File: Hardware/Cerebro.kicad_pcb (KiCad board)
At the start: 2 copper layers, 75 x 61.7 mm, 4 parts, among them U6 ATSAMD21G18A-AUT

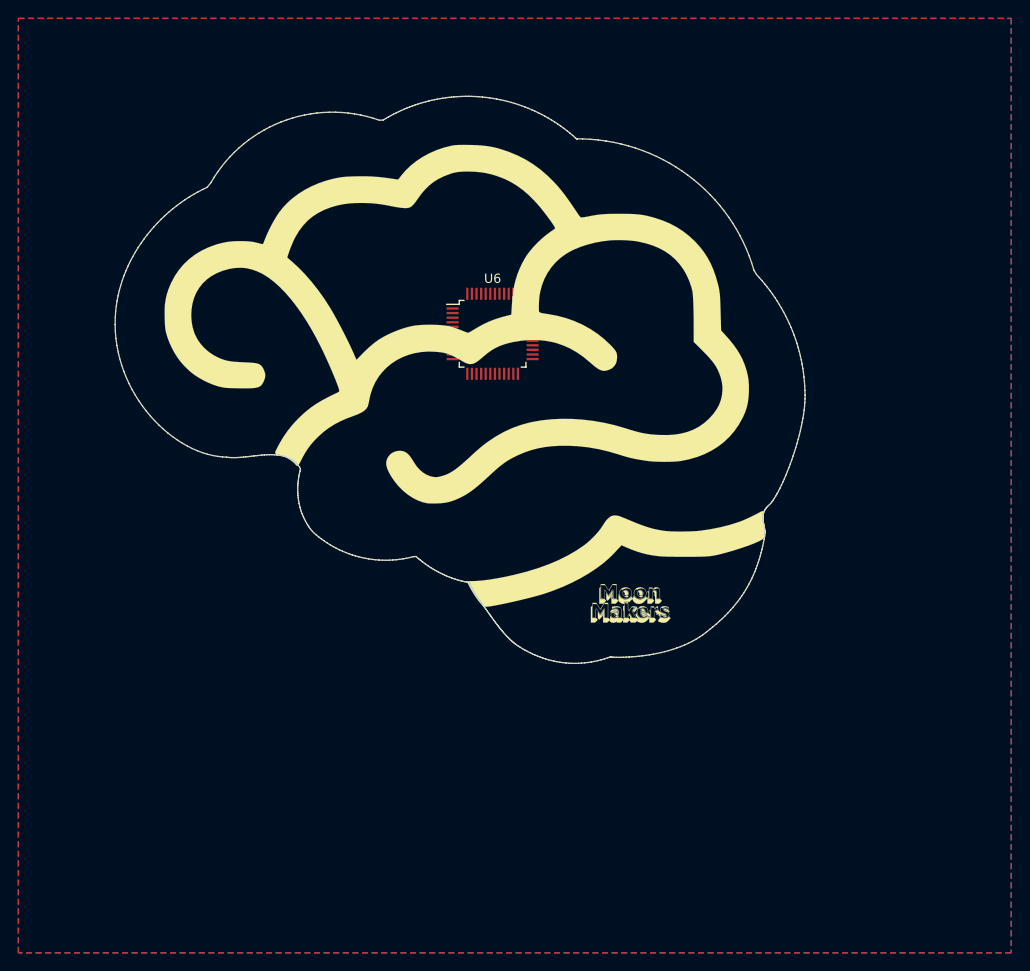
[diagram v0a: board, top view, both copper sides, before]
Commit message: update pcb
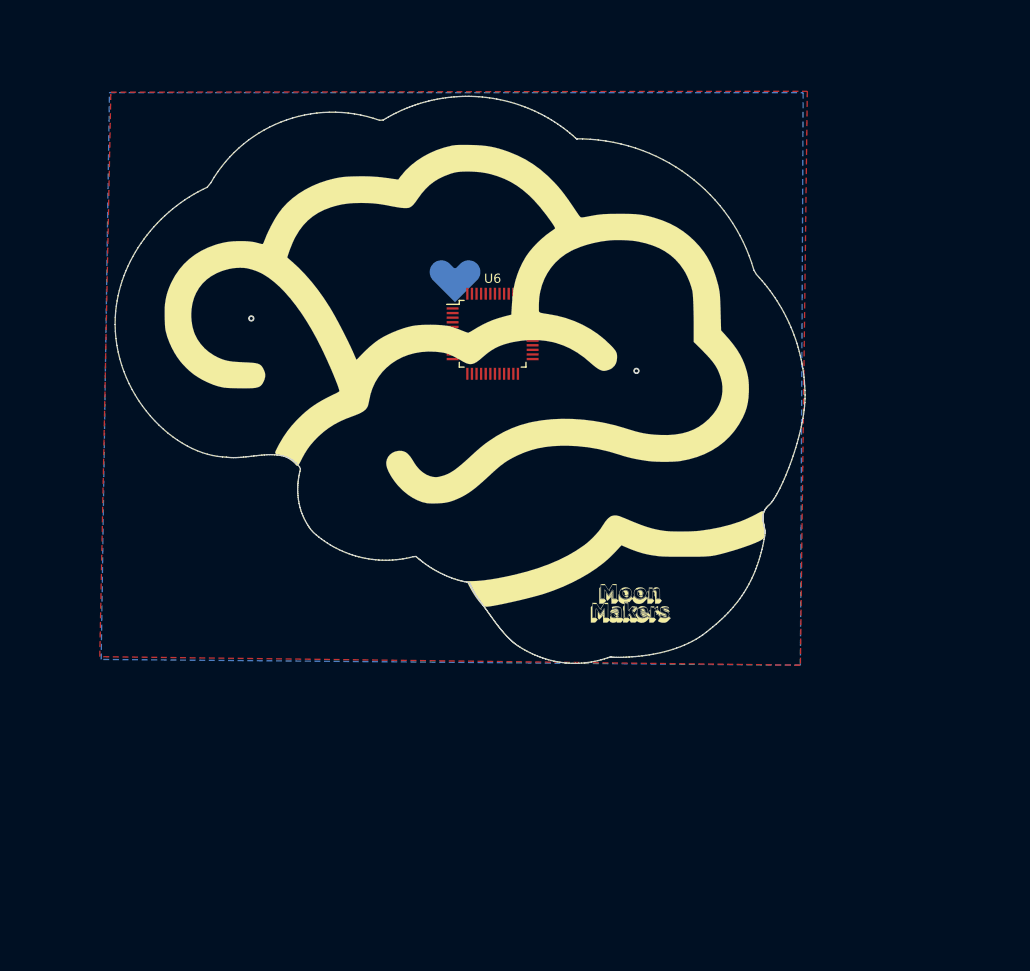
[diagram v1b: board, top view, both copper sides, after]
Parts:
- added svg2mod: G***, Aesthetics:heart, B.Cu at (142.7, 79.4)
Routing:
- net (no net): vias 0 -> 2
- added copper zone on B.Cu, net (none)
- added copper zone on F.Cu, net (none)
- removed copper zone on B.Cu, net GND
- removed copper zone on F.Cu, net GND
